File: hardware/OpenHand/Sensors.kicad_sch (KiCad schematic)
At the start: 6 parts, among them U5 ADS1115IDGS

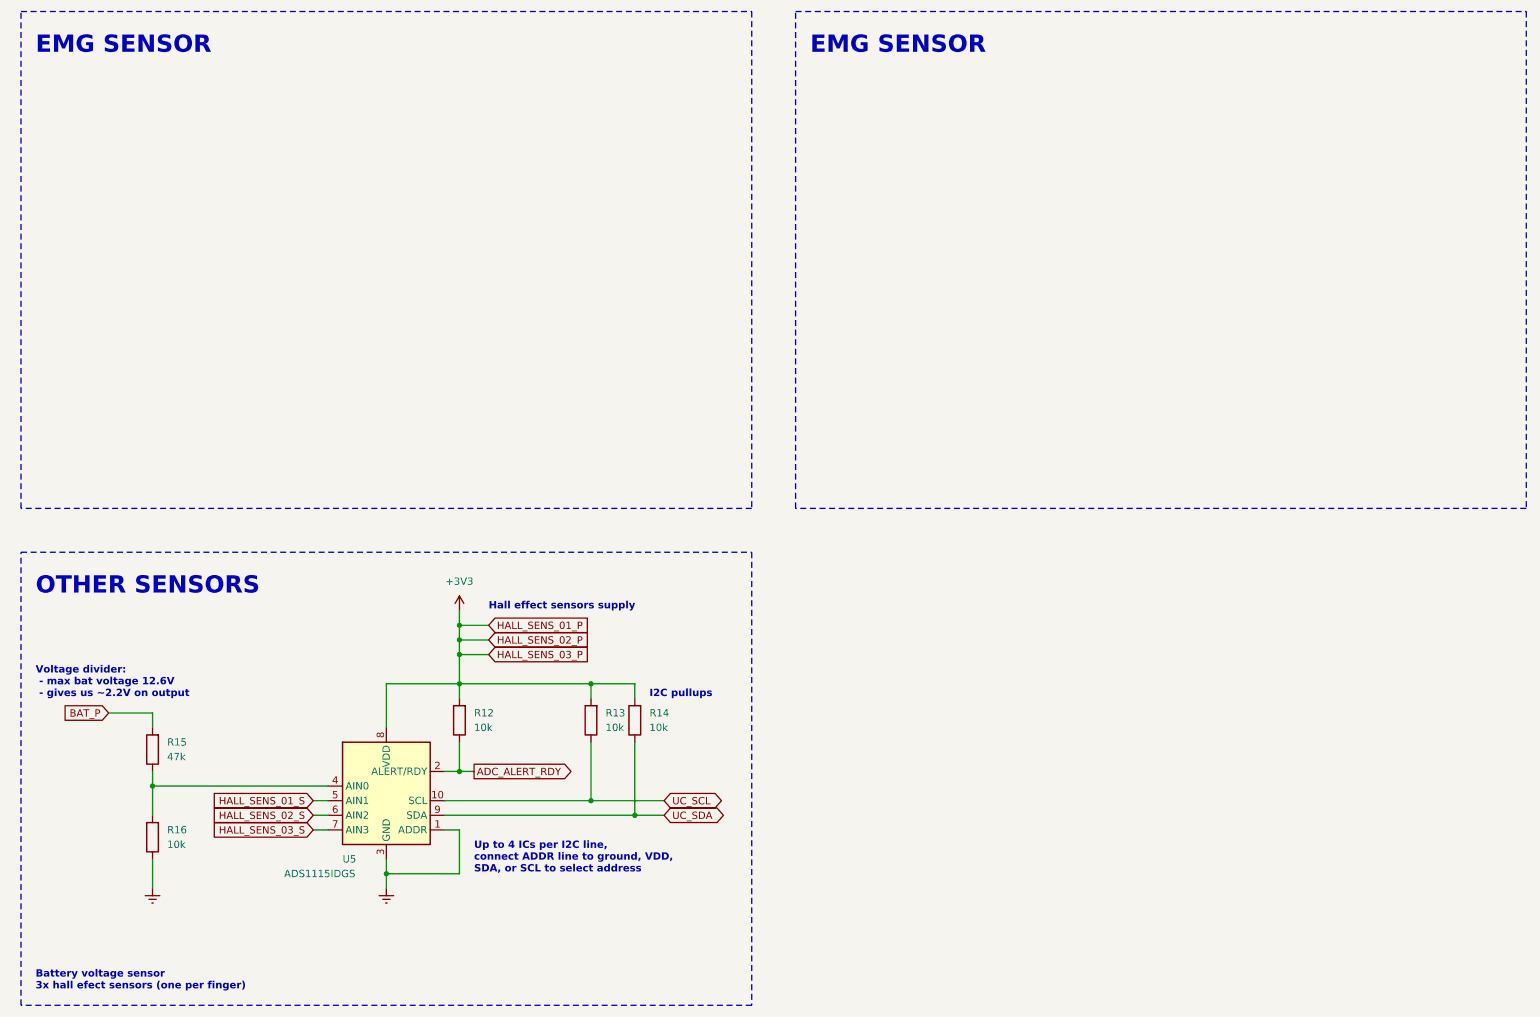
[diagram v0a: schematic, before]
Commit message: Update sch and board design
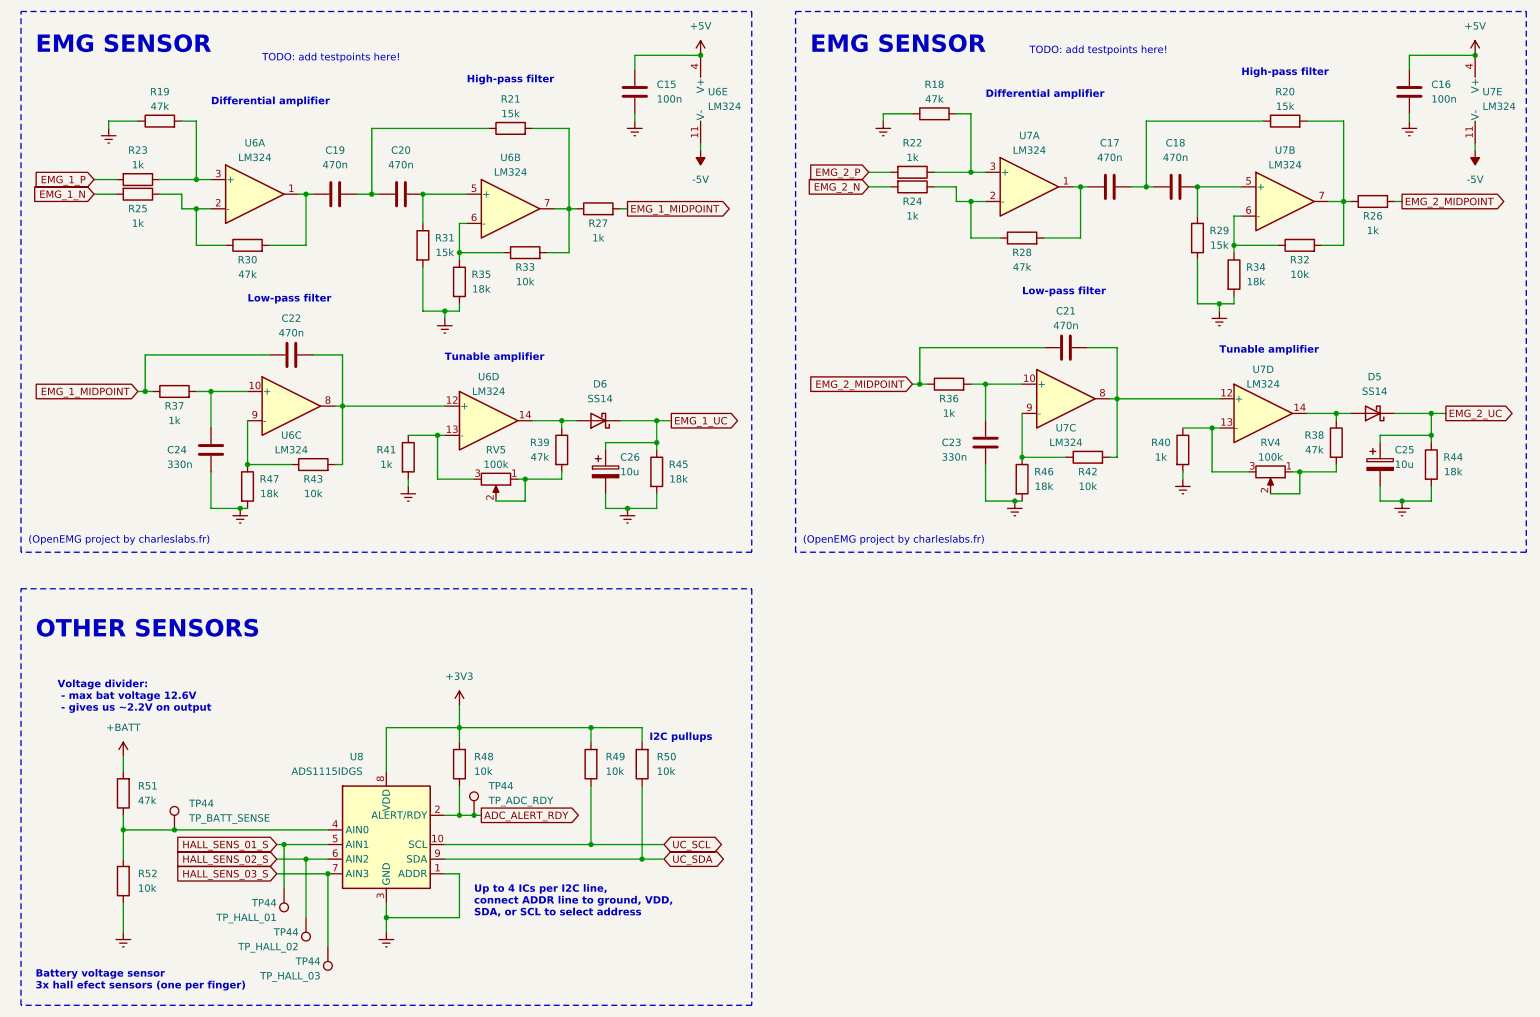
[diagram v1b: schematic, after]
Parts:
- added C15, C16: 100n, Capacitor_SMD:C_1206_3216Metric_Pad1.33x1.80mm_HandSolder, symbol Device:C
- added C17, C18, C19, C20, C21, C22: 470n, Capacitor_SMD:C_0805_2012Metric_Pad1.18x1.45mm_HandSolder, symbol Device:C
- added C23, C24: 330n, Capacitor_SMD:C_0805_2012Metric_Pad1.18x1.45mm_HandSolder, symbol Device:C
- added C25, C26: 10u, Capacitor_SMD:C_0805_2012Metric_Pad1.18x1.45mm_HandSolder, symbol Device:C_Polarized
- added D5, D6: SS14, Diode_SMD:D_SOD-123, symbol Device:D_Schottky
- added R18, R19, R28, R30, R38, R39: 47k, Resistor_SMD:R_0805_2012Metric_Pad1.20x1.40mm_HandSolder, symbol Device:R
- added R20, R21, R29, R31: 15k, Resistor_SMD:R_0805_2012Metric_Pad1.20x1.40mm_HandSolder, symbol Device:R
- added R22, R23, R24, R25, R26, R27, R36, R37, R40, R41: 1k, Resistor_SMD:R_0805_2012Metric_Pad1.20x1.40mm_HandSolder, symbol Device:R
- added R32, R33, R42, R43: 10k, Resistor_SMD:R_0805_2012Metric_Pad1.20x1.40mm_HandSolder, symbol Device:R
- added R34, R35, R44, R45, R46, R47: 18k, Resistor_SMD:R_0805_2012Metric_Pad1.20x1.40mm_HandSolder, symbol Device:R
- added RV4, RV5: 100k, Potentiometer_SMD:Potentiometer_Vishay_TS53YJ_Vertical, symbol Device:R_Potentiometer
- added TP44: TP_HALL_01, TestPoint:TestPoint_Pad_D1.0mm, symbol Connector:TestPoint
- added TP44: TP_BATT_SENSE, TestPoint:TestPoint_Pad_D1.0mm, symbol Connector:TestPoint
- added TP44: TP_ADC_RDY, TestPoint:TestPoint_Pad_D1.0mm, symbol Connector:TestPoint
- added TP44: TP_HALL_03, TestPoint:TestPoint_Pad_D1.0mm, symbol Connector:TestPoint
- added TP44: TP_HALL_02, TestPoint:TestPoint_Pad_D1.0mm, symbol Connector:TestPoint
- added U6, U7: LM324, Package_SO:SO-14_5.3x10.2mm_P1.27mm, symbol Amplifier_Operational:LM324
- R48: renamed from R12; footprint Resistor_SMD:R_1206_3216Metric -> Resistor_SMD:R_0805_2012Metric_Pad1.20x1.40mm_HandSolder
- R49: renamed from R13; footprint Resistor_SMD:R_1206_3216Metric -> Resistor_SMD:R_0805_2012Metric_Pad1.20x1.40mm_HandSolder
- R50: renamed from R14; footprint Resistor_SMD:R_1206_3216Metric -> Resistor_SMD:R_0805_2012Metric_Pad1.20x1.40mm_HandSolder
- R51: renamed from R15; footprint Resistor_SMD:R_1206_3216Metric -> Resistor_SMD:R_0805_2012Metric_Pad1.20x1.40mm_HandSolder
- R52: renamed from R16; footprint Resistor_SMD:R_1206_3216Metric -> Resistor_SMD:R_0805_2012Metric_Pad1.20x1.40mm_HandSolder
- renumbered U5 to U8
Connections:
- net ADC_ALERT_RDY: now also TP44.1
- net Earth: now also C15.2, C16.2, C23.1, C24.1, C25.2, C26.2, R18.1, R19.1, R29.2, R31.2, R34.2, R35.2, R40.2, R41.2, R44.2, R45.2, R46.2, R47.2
- net HALL_SENS_01_S: now also TP44.1
- net HALL_SENS_02_S: now also TP44.1
- net HALL_SENS_03_S: now also TP44.1
- net at R51.1, R52.2, U8.4 (AIN0): now also TP44.1
- net BAT_P renamed +BATT
- new net: C21.2, R42.2, U7.12 (+), U7.8
- new net: R40.1, RV4.3, U7.13 (-)
- new net: D5.2 (A), R38.1, U7.14
- new net: R41.1, RV5.3, U6.13 (-)
- new net: C23.2, R36.2, U7.10 (+)
- new net: C24.2, R37.2, U6.10 (+)
- new net: C22.2, R43.2, U6.12 (+), U6.8
- new net: R43.1, R47.1, U6.9 (-)
- new net: R42.1, R46.1, U7.9 (-)
- new net: R21.2, R27.1, R33.2, U6.7
- new net: R33.1, R35.1, U6.6 (-)
- new net: D6.2 (A), R39.1, U6.14
- new net: C17.1, R28.2, U7.1
- new net: R24.1, R28.1, U7.2 (-)
- new net: R18.2, R22.1, U7.3 (+)
- new net: C20.2, R31.1, U6.5 (+)
- new net: C17.2, C18.1, R20.1
- new net: C18.2, R29.1, U7.5 (+)
- new net: C19.1, R30.2, U6.1
- new net: R25.1, R30.1, U6.2 (-)
- new net: R19.2, R23.1, U6.3 (+)
- new net: R39.2, RV5.1, RV5.2
- new net: R20.2, R26.1, R32.2, U7.7
- new net: R32.1, R34.1, U7.6 (-)
- new net: C19.2, C20.1, R21.1
- new net: R38.2, RV4.1, RV4.2
- new net +5V: C15.1, C16.1, U6.4 (V+), U7.4 (V+)
- new net -5V: U6.11 (V-), U7.11 (V-)
- new net EMG_1_MIDPOINT: C22.1, R27.2, R37.1
- new net EMG_1_N: R25.2
- new net EMG_1_P: R23.2
- new net EMG_1_UC: C26.1, D6.1 (K), R45.1
- new net EMG_2_MIDPOINT: C21.1, R26.2, R36.1
- new net EMG_2_N: R24.2
- new net EMG_2_P: R22.2
- new net EMG_2_UC: C25.1, D5.1 (K), R44.1
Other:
- note added: "(OpenEMG project by charleslabs.fr)"
- note added: "Differential amplifier"
- note added: "High-pass filter"
- note added: "Low-pass filter"
- note added: "TODO: add testpoints here!"
- note added: "Tunable amplifier"
- note removed: "Hall effect sensors supply"
- moved on the sheet: R48, R49, R50, R51, R52, U8
